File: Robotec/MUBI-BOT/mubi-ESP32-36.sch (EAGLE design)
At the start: 22 parts, among them IC1 L293D, IC2 7805T

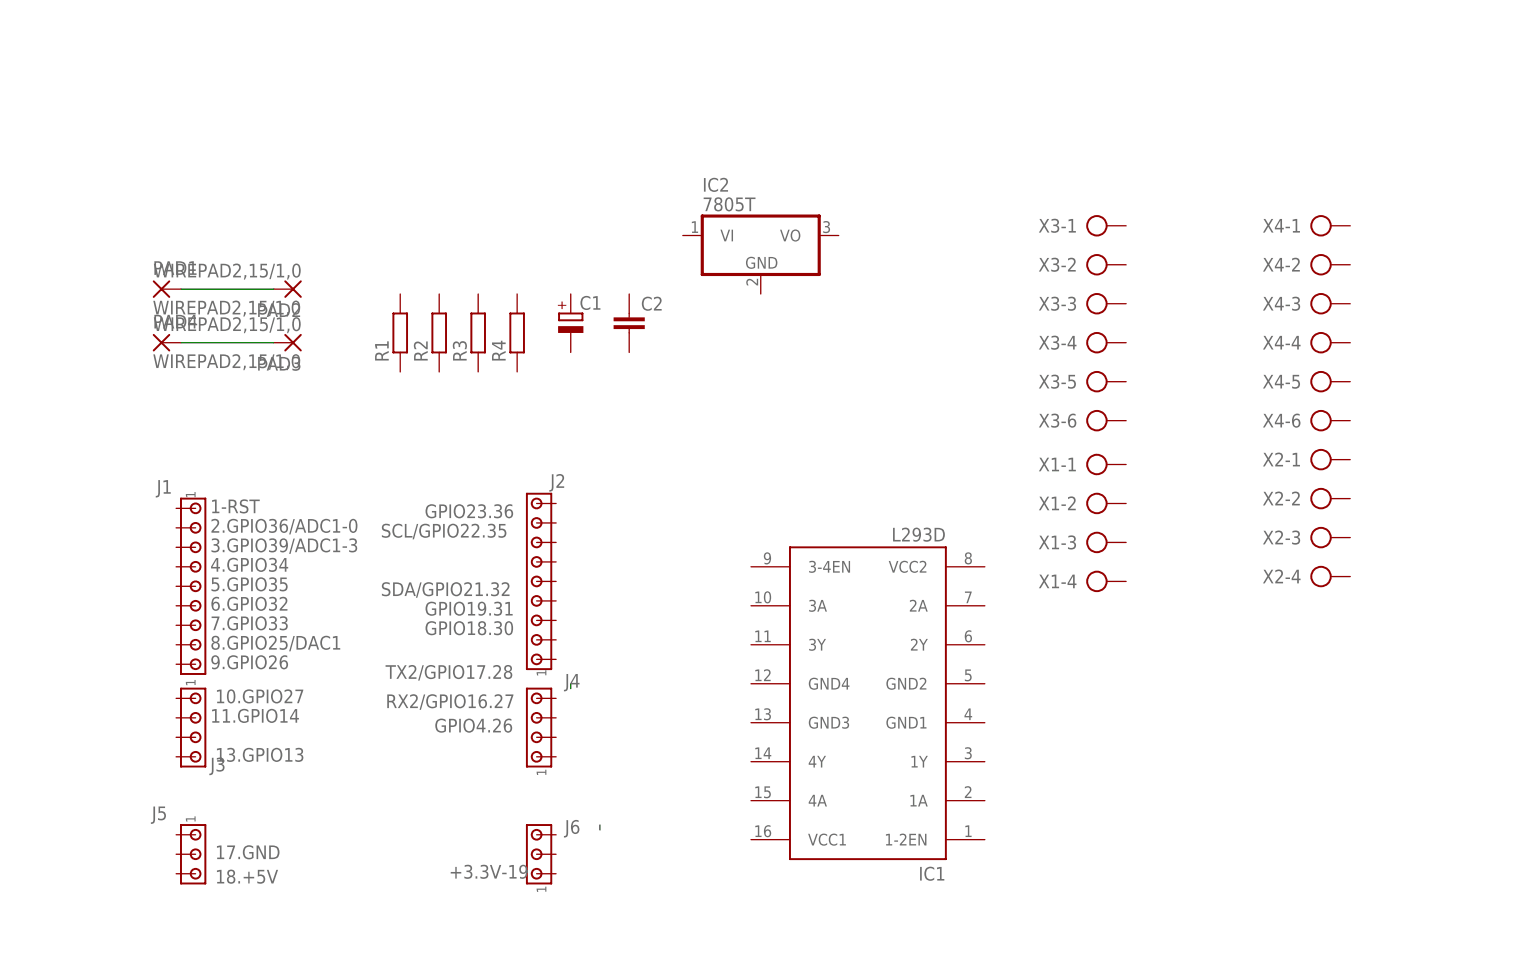
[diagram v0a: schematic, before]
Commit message: update MUBI-BOT
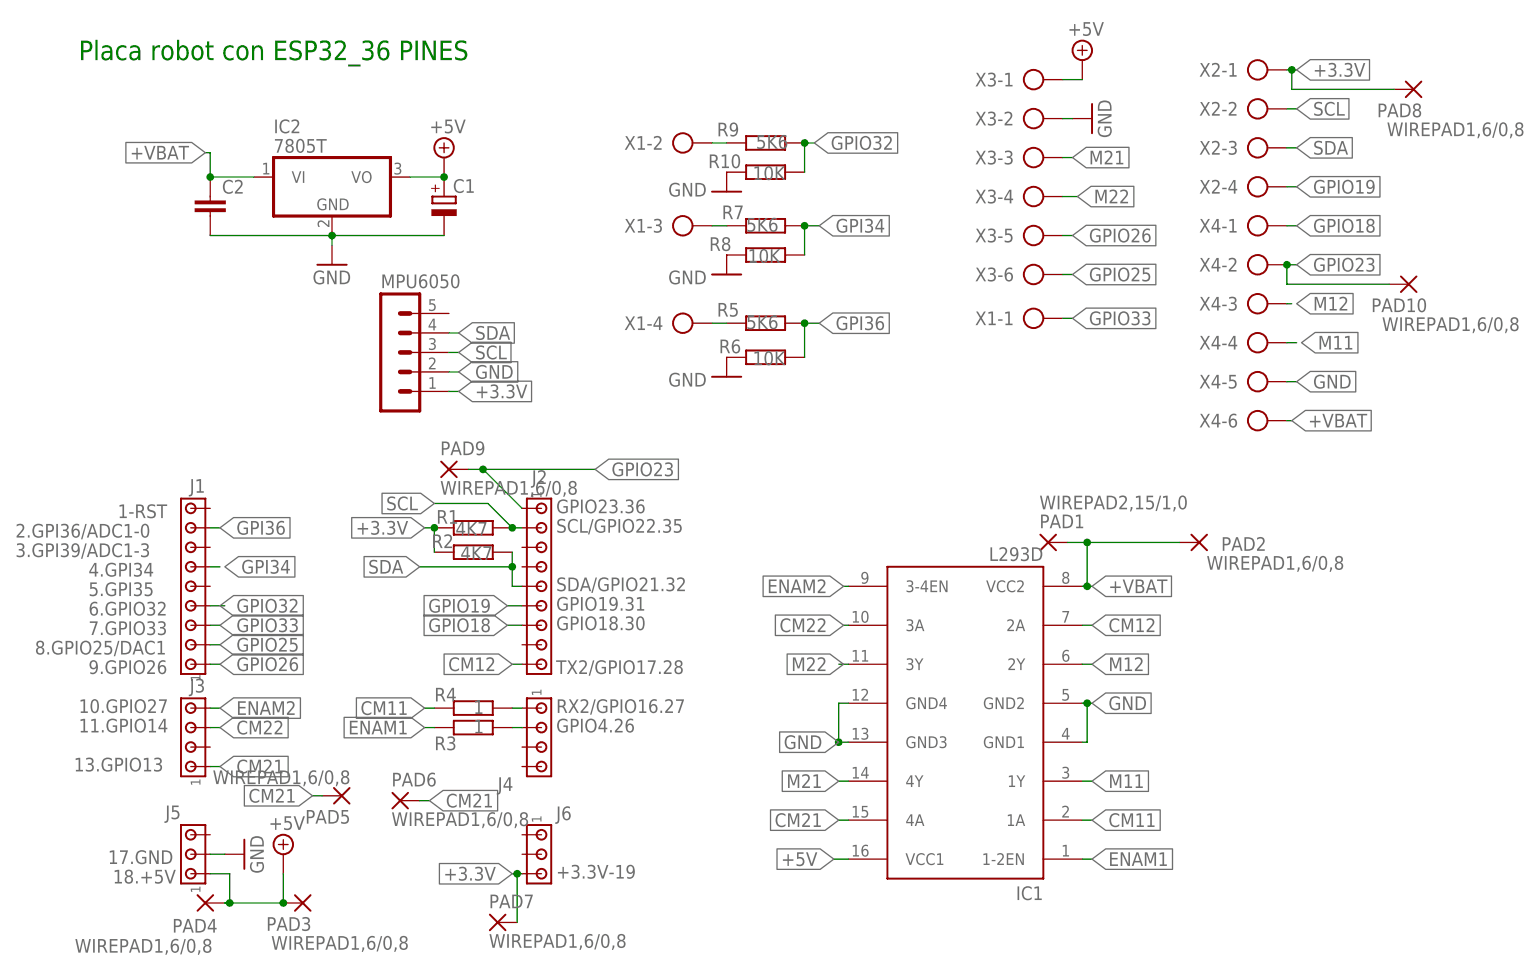
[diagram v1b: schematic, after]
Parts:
- added MPU6050: (no value), con-lstb:MA05-1
- added PAD10, PAD5, PAD6, PAD7, PAD8, PAD9: WIREPAD1,6/0,8, wirepad:WIREPAD1,6/0,8
- added R10, R6, R8: 10K, resistor:R-EU_0204/5
- added R5, R7, R9: 5K6, resistor:R-EU_0204/5
- PAD2, PAD3, PAD4: value WIREPAD2,15/1,0 -> WIREPAD1,6/0,8; device wirepad:WIREPAD2,15/1,0 -> wirepad:WIREPAD1,6/0,8
- R1, R2: value (none) -> 4K7; device resistor:R-EU_0207/10 -> rcl:R-EU_0207/7
- R3, R4: value (none) -> 1
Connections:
- new net +3.3V: J6.3, MPU6050.1, PAD7.P, PAD8.P, R1.2, R2.2, X2-1.KL
- new net +5V: C1.+, IC1.VCC1, IC2.VO, J5.1, PAD3.P, PAD4.P, X3-1.KL
- new net +VBAT: C2.1, IC1.VCC2, IC2.VI, PAD1.P, PAD2.P, X4-6.KL
- new net CM11: IC1.1A, R4.1
- new net CM12: IC1.2A, J2.9
- new net CM21: IC1.4A, J3.1, PAD5.P, PAD6.P
- new net CM22: IC1.3A, J3.3
- new net ENAM1: IC1.1-2EN, R3.1
- new net ENAM2: IC1.3-4EN, J3.4
- new net GND: C1.-, C2.2, IC1.GND1, IC1.GND2, IC1.GND3, IC1.GND4, IC2.GND, J5.2, MPU6050.2, R10.2, R6.2, R8.2, X3-2.KL, X4-5.KL
- new net GPI34: J1.6, R7.2, R8.1
- new net GPI36: J1.8, R5.2, R6.1
- new net GPIO18: J2.7, X4-1.KL
- new net GPIO19: J2.6, X2-4.KL
- new net GPIO23: J2.1, PAD10.P, PAD9.P, X4-2.KL
- new net GPIO25: J1.2, X3-6.KL
- new net GPIO26: J1.1, X3-5.KL
- new net GPIO32: J1.4, R10.1, R9.2
- new net GPIO33: J1.3, X1-1.KL
- new net M11: IC1.1Y, X4-4.KL
- new net M12: IC1.2Y, X4-3.KL
- new net M21: IC1.4Y, X3-3.KL
- new net M22: IC1.3Y, X3-4.KL
- new net N$3: R5.1, X1-4.KL
- new net N$5: R7.1, X1-3.KL
- new net N$8: R9.1, X1-2.KL
- new net SCL: J2.2, MPU6050.3, R1.1, X2-2.KL
- new net SDA: J2.5, MPU6050.4, R2.1, X2-3.KL
- net N$1: now also J4.2, R3.2; no longer PAD1.P, PAD2.P
- net N$2: now also J4.1, R4.2; no longer PAD3.P, PAD4.P
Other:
- note added: "2.GPI36/ADC1-0"
- note added: "3.GPI39/ADC1-3"
- note added: "4.GPI34"
- note added: "5.GPI35"
- note added: "Placa robot con ESP32_36 PINES"
- note removed: "2.GPIO36/ADC1-0"
- note removed: "3.GPIO39/ADC1-3"
- note removed: "4.GPIO34"
- note removed: "5.GPIO35"
- moved on the sheet: C1, C2, IC1, IC2, J1, J2, J3, J4, J5, J6, PAD1, PAD2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
